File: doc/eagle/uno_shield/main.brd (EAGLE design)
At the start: 58.7 x 58.4 mm, 15 parts, among them U1 ARDUINOR3-BPLACE

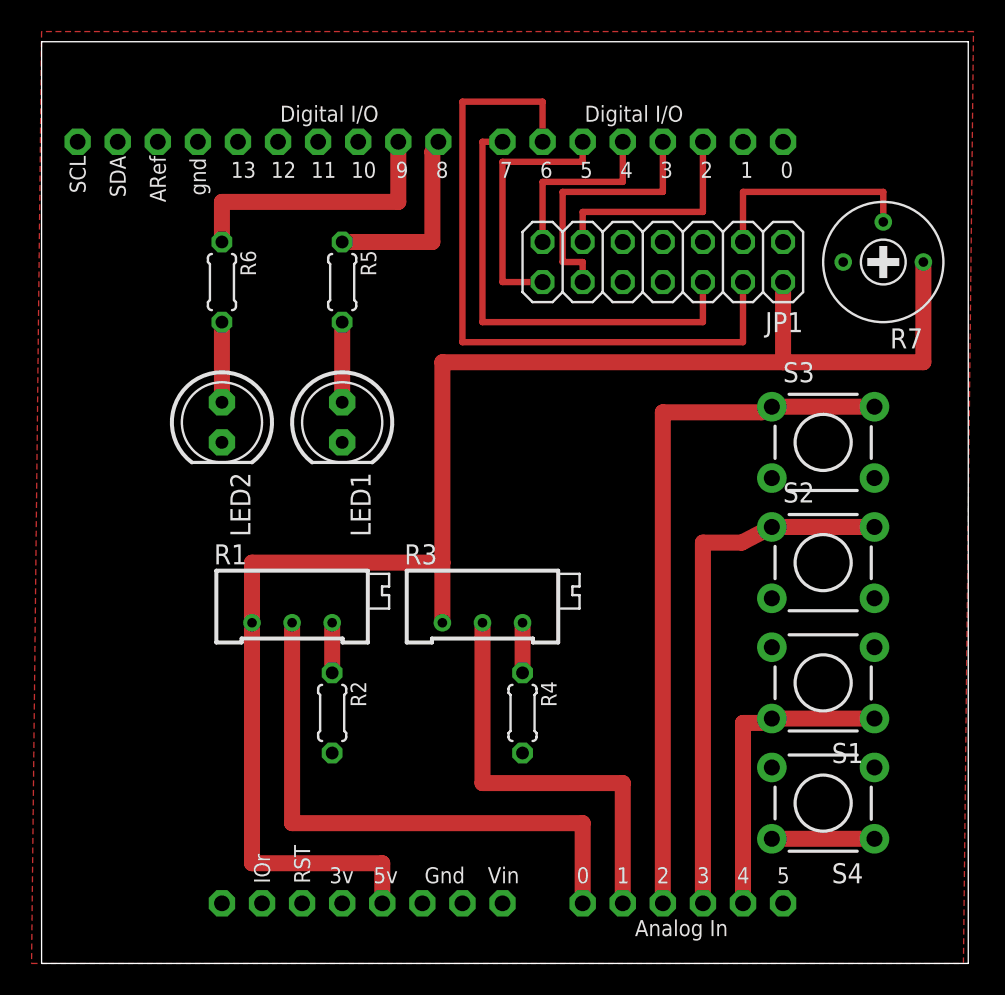
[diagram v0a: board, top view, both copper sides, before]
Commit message: [ add ] routed board, main.png
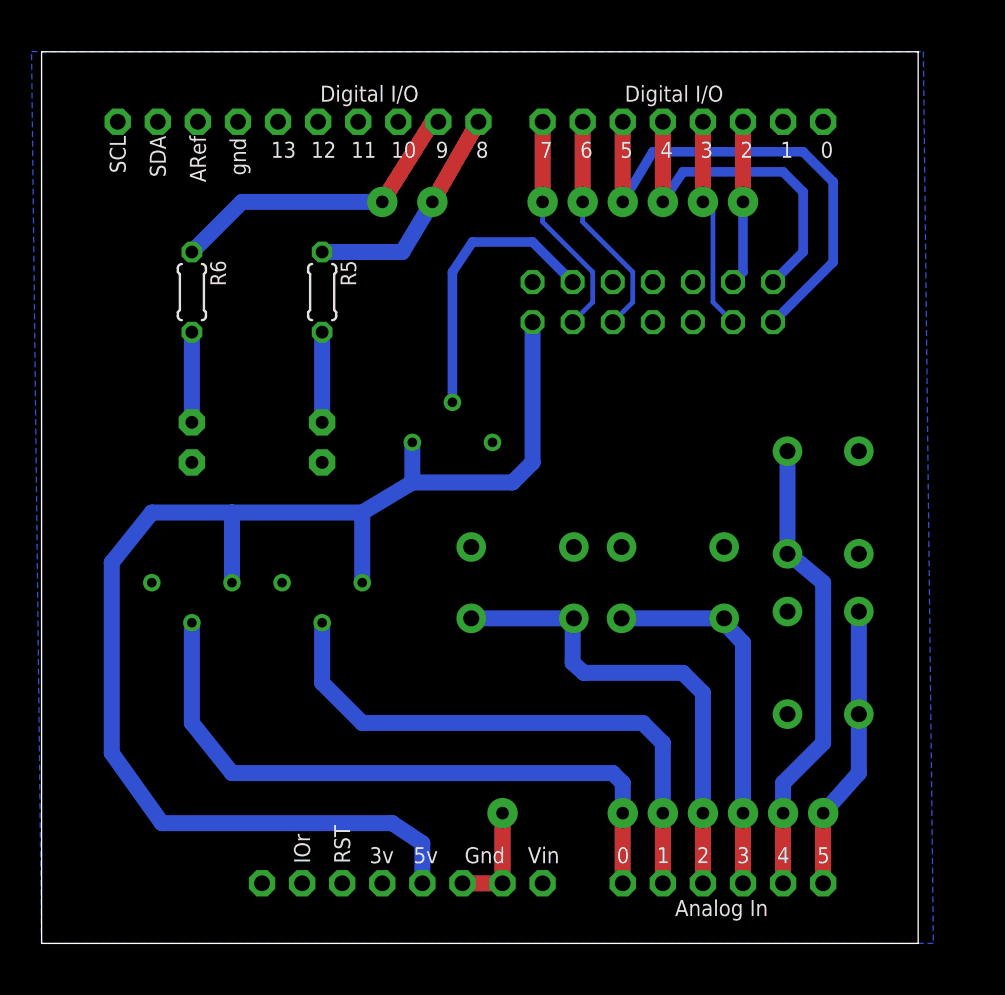
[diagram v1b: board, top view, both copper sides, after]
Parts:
- removed R2, R4: 1k, rcl:0204/5
- removed R3: (no value), rcl:RTRIM64X
- added R8: (no value), resistor:RTRIM3339P
- R1: device rcl:RTRIM64X -> resistor:RTRIM3339P
- moved R7 29.6 mm to (26.0, 31.8), flipped to the bottom
- moved S3 21.0 mm to (30.5, 22.9), flipped to the bottom, turned to 180 degrees
- moved S1 11.4 mm to (49.5, 27.9), flipped to the bottom, turned to 270 degrees
- moved S2 9.61 mm to (40.0, 22.9), flipped to the bottom, turned to 180 degrees
- moved S4 8.89 mm to (49.5, 17.8), flipped to the bottom, turned to 90 degrees
- moved U1 2.84 mm to (-14.0, 1.27)
- moved JP1 2.62 mm to (38.7, 40.6), flipped to the bottom
- moved R1 2.29 mm to (17.8, 22.9), flipped to the bottom, turned to 0 degrees
- moved LED2 2.29 mm to (9.53, 31.8), flipped to the bottom
- moved R6 2.01 mm to (9.53, 41.3)
- moved LED1 1.80 mm to (17.8, 31.8), flipped to the bottom
- moved R5 1.42 mm to (17.8, 41.3)
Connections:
- removed net N$1: R1.3, R2.1
- removed net N$2: R3.3, R4.1
- net ADC_VCAP: now also R8.2; no longer R1.2
- net ADC_VOUT: now also R1.2; no longer R3.2
- net BUT_MINUS: now also S4.1, S4.2, U1.A5; no longer S2.1, S2.2, U1.A3
- net BUT_MODE: now also S2.1, S2.2, U1.A3; no longer S1.1, S1.2, U1.A4
- net BUT_PLUS: now also S1.1, S1.2, U1.A4; no longer S3.1, S3.2, U1.A2
- net BUT_SAVE: now also S3.1, S3.2, U1.A2; no longer S4.1, S4.2, U1.A5
- net GND: now also R1.3, R8.3; no longer R2.2, R4.2
- net LCD_EN: now also U1.D6; no longer U1.D7
- net LCD_RS: now also U1.D7; no longer U1.D6
- net UNO_5V: now also R8.1; no longer R3.1
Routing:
- net LCD_RS: track 44.5 -> 14.5 mm, vias 0 -> 1
- net BUT_SAVE: track 6.50 -> 30.4 mm, vias 0 -> 1
- net BUT_MINUS: track 34.0 -> 18.1 mm, vias 0 -> 1
- net BUT_PLUS: track 44.6 -> 29.5 mm, vias 0 -> 1
- net LCD_DB7: track 16.5 -> 31.5 mm, vias 0 -> 1
- net LCD_EN: track 29.2 -> 14.5 mm, vias 0 -> 1
- net UNO_5V: track 100.3 -> 86.5 mm
- net LCD_DB6: track 11.4 -> 22.0 mm, vias 0 -> 1
- net ADC_VOUT: track 26.7 -> 35.9 mm, vias 0 -> 1
- net GND: track 0.00 -> 6.98 mm, vias 0 -> 1
- net ADC_VCAP: track 36.2 -> 41.8 mm, vias 0 -> 1
- net LCD_VO: track 14.0 -> 17.9 mm
- net BUT_MODE: track 20.0 -> 23.8 mm, vias 0 -> 1
- net LCD_DB4: track 14.0 -> 10.4 mm, vias 0 -> 1
- net N$2: track 3.18 -> 0.00 mm
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- added copper zone on layer 16, net GND
- removed copper zone on layer 1, net GND
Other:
- board size 58.7 x 58.4 mm -> 55.5 x 56.5 mm
